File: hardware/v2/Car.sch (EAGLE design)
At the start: 64 parts

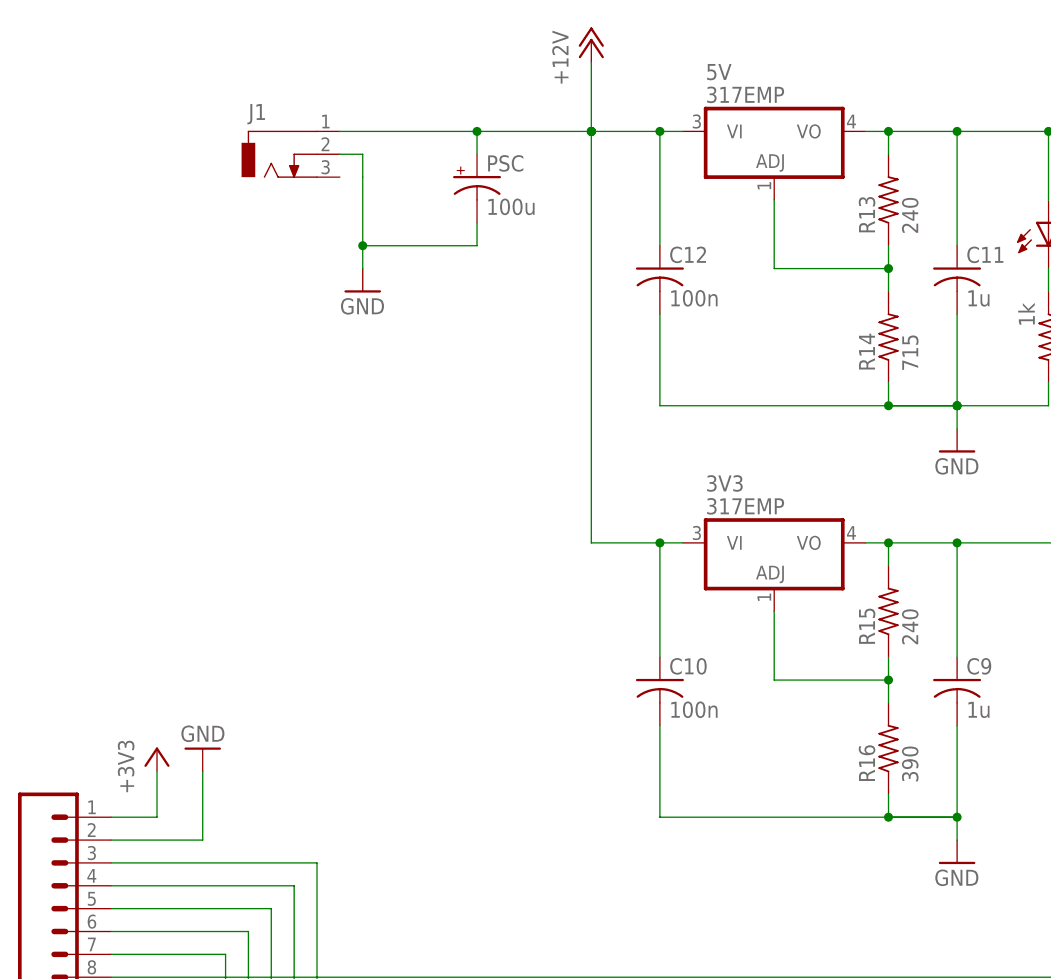
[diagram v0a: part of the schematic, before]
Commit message: Minor cleanup.
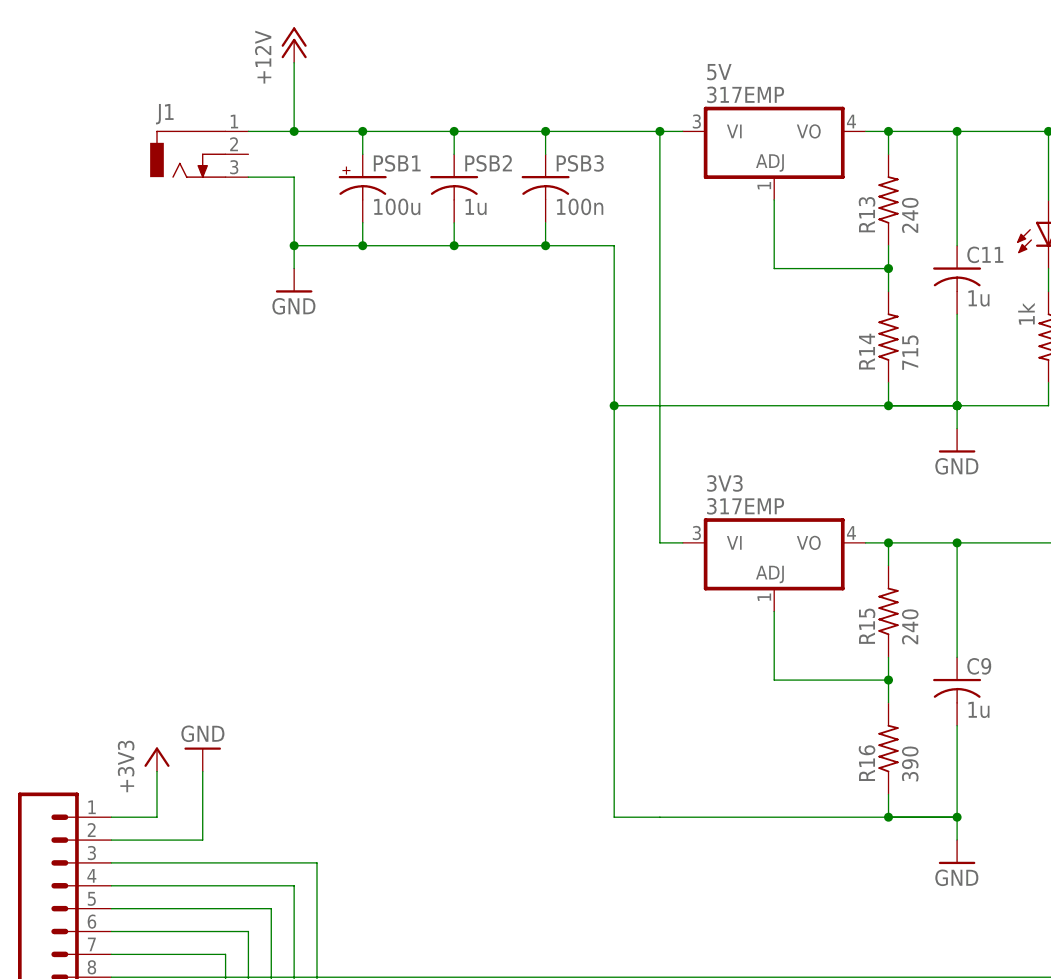
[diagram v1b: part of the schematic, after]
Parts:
- removed C10, C12: 100n, rcl:C-USC0805
- removed PSC: 100u, SparkFun-Passives:CAP_POLC
- added PSB1: 100u, SparkFun-Passives:CAP_POLC
- added PSB2: 1u, rcl:C-USC0805
- added PSB3: 100n, rcl:C-USC0805
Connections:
- net +12V: now also PSB1.+, PSB2.1, PSB3.1; no longer C10.1, C12.1, PSC.+
- net GND: now also J1.3, PSB1.-, PSB2.2, PSB3.2; no longer C10.2, C12.2, J1.2, PSC.-
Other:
- moved on the sheet: J1
